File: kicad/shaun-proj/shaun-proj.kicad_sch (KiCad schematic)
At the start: 1 part

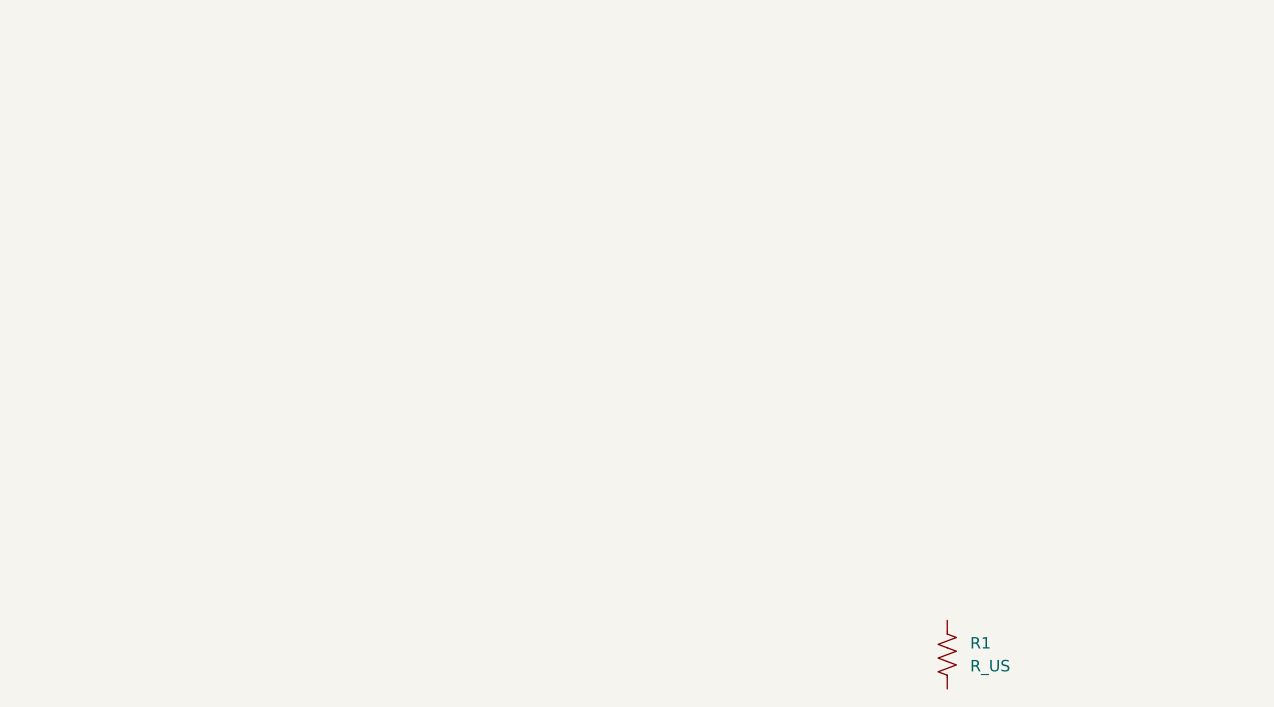
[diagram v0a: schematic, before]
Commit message: 9v usb req
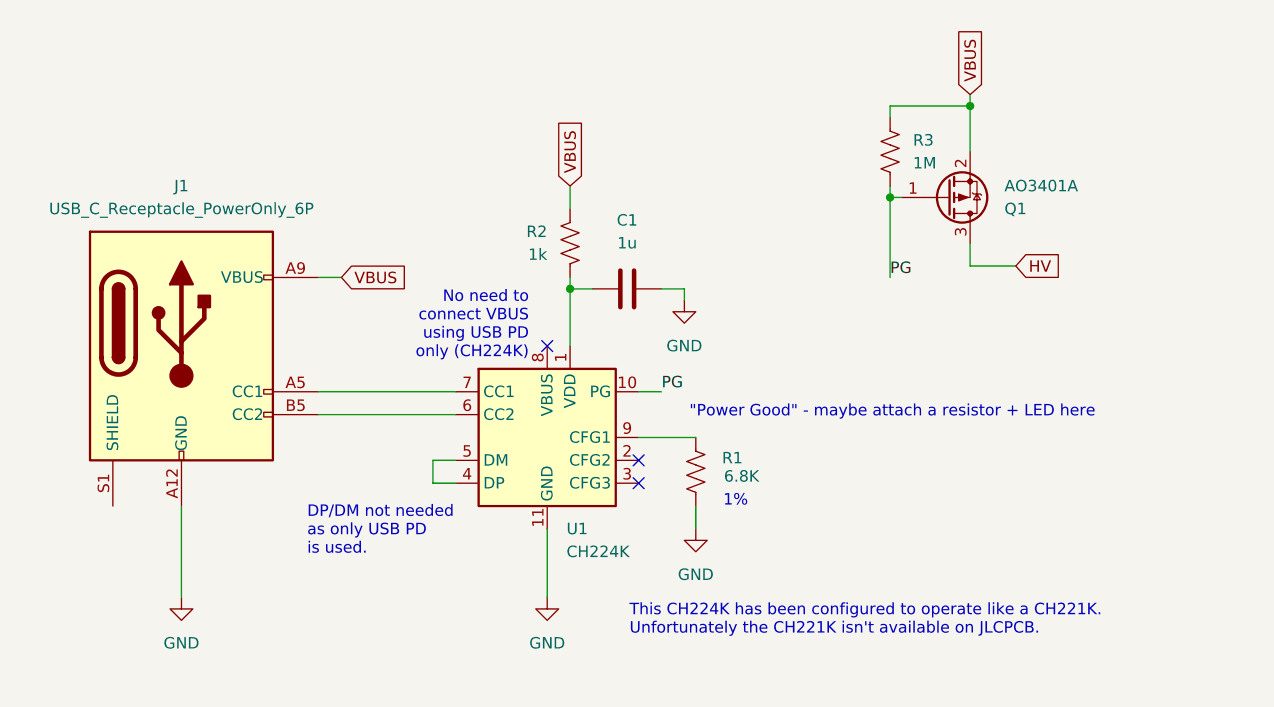
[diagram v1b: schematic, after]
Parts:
- added C1: 1u, symbol Device:C
- added J1: USB_C_Receptacle_PowerOnly_6P, symbol Connector:USB_C_Receptacle_PowerOnly_6P
- added Q1: AO3401A, Package_TO_SOT_SMD:SOT-23, symbol Transistor_FET:AO3401A
- added R2: 1k, symbol Device:R_US
- added R3: 1M, Resistor_SMD:R_0603_1608Metric, symbol Device:R_US
- added U1: CH224K, Package_SO:SSOP-10-1EP_3.9x4.9mm_P1mm_EP2.1x3.3mm, symbol Interface_USB:CH224K
- R1: value R_US -> 6.8K; footprint (none) -> Resistor_SMD:R_0603_1608Metric
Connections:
- net GND: now reaches R1.1
- net GND: now also C1.2, J1.A12 (GND), J1.B12 (GND), U1.11 (GND)
- net at R1.2: now also U1.9 (CFG1)
- new net: C1.1, R2.1, U1.1 (VDD)
- new net: U1.4 (DP), U1.5 (DM)
- new net: J1.B5 (CC2), U1.6 (CC2)
- new net: J1.A5 (CC1), U1.7 (CC1)
- new net HV: Q1.3 (D)
- new net PG: Q1.1 (G), R3.2, U1.10 (PG)
- new net VBUS: J1.A9 (VBUS), J1.B9 (VBUS), Q1.2 (S), R2.2, R3.1
- no-connect marks 0 -> 3
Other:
- note added: ""Power Good" - maybe attach a resistor + LED here"
- note added: "1%"
- note added: "DP/DM not needed as only USB PD is used."
- note added: "No need to connect VBUS using USB PD only (CH224K)"
- note added: "This CH224K has been configured to operate like a CH221K. Unfortunately the CH221K isn't available on JLCPCB."
